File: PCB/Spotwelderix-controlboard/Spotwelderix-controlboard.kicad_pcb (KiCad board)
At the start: 2 copper layers, 83 x 60 mm, 42 parts, among them J2 LEDs, J3 Switch_OnOFF, J4 Int_Charger_supply, P1 Display, P2 CONN_01X08, Q1 DMG1012T-7, Q2 DMG1012T-7, Q3 DMG1012T-7, Q4 DMG1012T-7, U1 NodeMCU32, U2 ADS1115_Module, U3 LM7805M_TO263

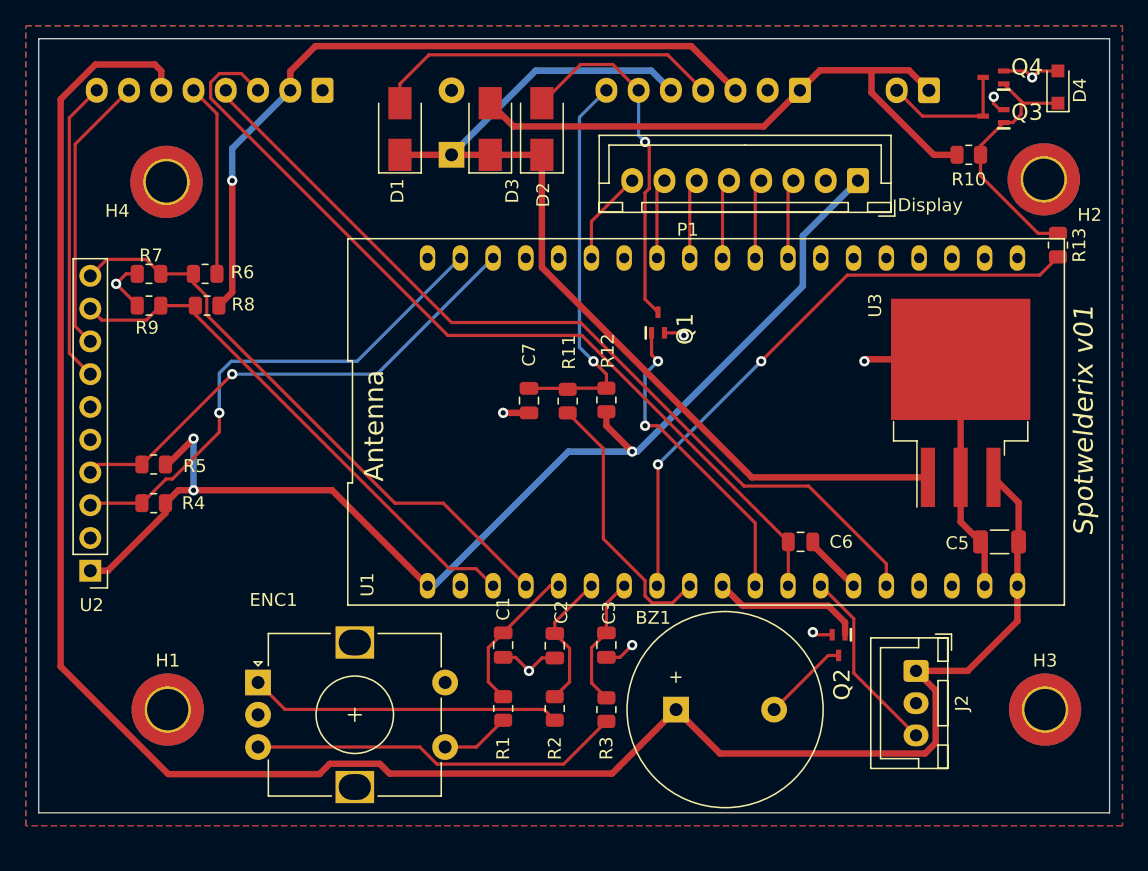
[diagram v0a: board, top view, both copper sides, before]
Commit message: ordered version v01
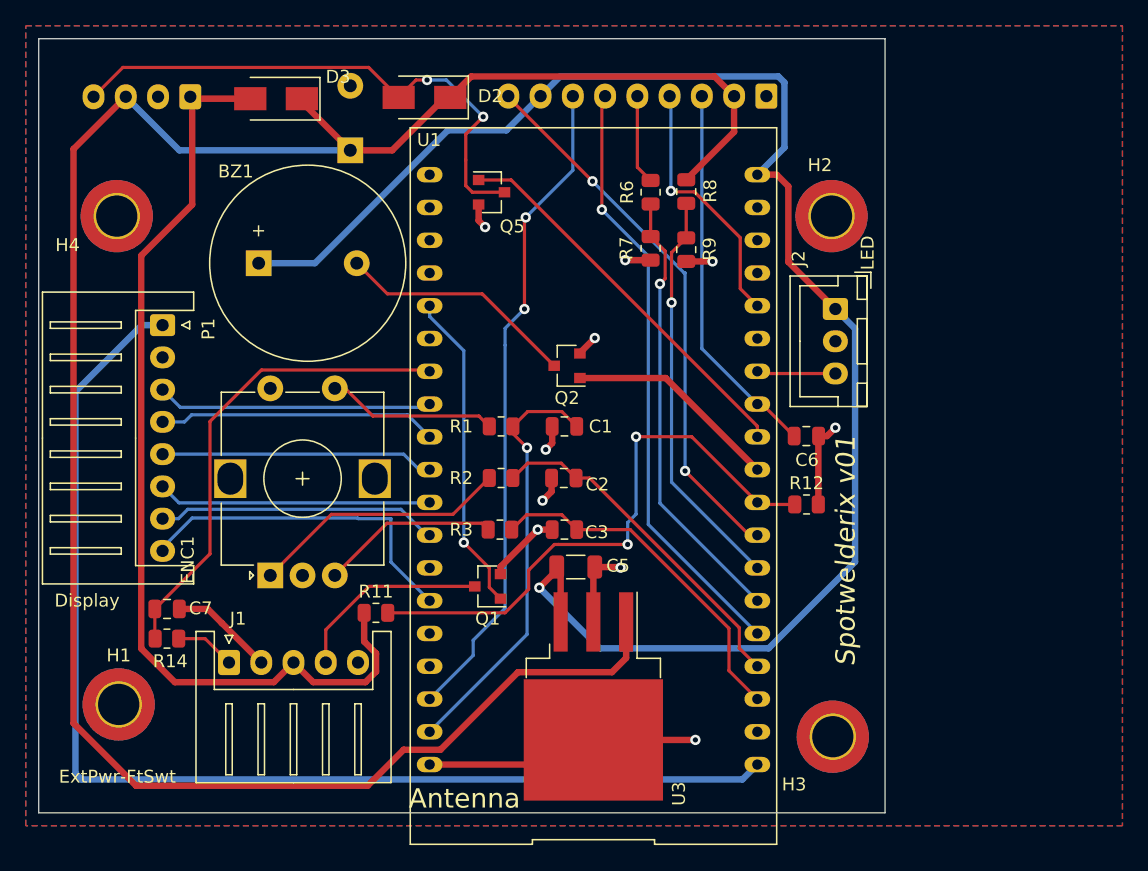
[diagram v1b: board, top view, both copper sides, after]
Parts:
- removed D1: D, Diode_SMD:D_SMA
- removed D4: 3.6V, Diode_SMD:D_SOD-323_HandSoldering
- removed J4: Int_Charger_supply, Connector_JST:JST_XH_B2B-XH-A_1x02_P2.50mm_Vertical
- removed Q3, Q4: DMG1012T-7, SamacSys_Parts:SOT50P160X80-3N
- removed R10: 10k, Resistor_SMD:R_0805_2012Metric
- removed R13: 100, Resistor_SMD:R_0805_2012Metric
- removed R4, R5: 3k3, Resistor_SMD:R_0805_2012Metric
- removed U2: ADS1115_Module, Connector_PinHeader_2.54mm:PinHeader_1x10_P2.54mm_Vertical
- added J1: ChargerPower, Connector_JST:JST_XH_S5B-XH-A_1x05_P2.50mm_Horizontal, F.Cu at (34.8, 68.3)
- added Q5: AO3400A, Package_TO_SOT_SMD:SOT-23, F.Cu at (55.1, 31.9)
- added R14: 100, Resistor_SMD:R_0805_2012Metric, F.Cu at (29.9, 66.5)
- C7: value 100n -> 100p
- J3: value Switch_OnOFF -> ExtPwr_FAn; footprint Connector_JST:JST_XH_B7B-XH-A_1x07_P2.50mm_Vertical -> Connector_JST:JST_XH_B4B-XH-A_1x04_P2.50mm_Vertical
- P1: footprint Connector_JST:JST_XH_B8B-XH-A_1x08_P2.50mm_Vertical -> Connector_JST:JST_XH_S8B-XH-A_1x08_P2.50mm_Horizontal
- P2: value CONN_01X08 -> PowerPCB; footprint Connector_JST:JST_XH_B8B-XH-A_1x08_P2.50mm_Vertical -> Connector_JST:JST_XH_B9B-XH-A_1x09_P2.50mm_Vertical
- Q1, Q2: value DMG1012T-7 -> AO3400A; footprint SamacSys_Parts:SOT50P160X80-3N -> Package_TO_SOT_SMD:SOT-23
- R11: value 100 -> 33k
- moved P1 55.1 mm to (29.6, 42.2), turned to 270 degrees
- moved BZ1 47.4 mm to (37.0, 37.4)
- moved J3 47.3 mm to (31.8, 24.5)
- moved R9 41.9 mm to (70.2, 36.3), turned to 270 degrees
- moved R7 38.9 mm to (67.4, 36.2), turned to 270 degrees
- moved R8 38.2 mm to (70.2, 31.8), turned to 270 degrees
- moved U3 36.4 mm to (63.0, 71.0), turned to 270 degrees
- moved R6 35.1 mm to (67.4, 31.9), turned to 270 degrees
- moved P2 34.4 mm to (76.4, 24.4)
- moved C5 32.9 mm to (61.6, 61.0), turned to 0 degrees
- moved C7 32.4 mm to (29.9, 64.2), turned to 0 degrees
- moved Q2 30.2 mm to (61.0, 45.4), turned to 180 degrees
- moved J2 28.7 mm to (81.8, 41.0)
- moved Q1 24.3 mm to (54.8, 62.5), turned to 180 degrees
- moved R11 22.1 mm to (46.1, 64.5), turned to 0 degrees
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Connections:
- C4 pad 1: /LM7805_in -> VCC
- C7 pad 1: Net-(C7-Pad1) -> FootSwitch
- D2 pad 1: /LM7805_in -> VCC
- D3 pad 1: /LM7805_in -> VCC
- J3 pad 4: Net-(D1-Pad2) -> FAN_GND
- P2 pad 6: +5V -> Vbat_ADC
- P2 pad 7: R_Schunt_H -> EnableSupply
- P2 pad 8: R_Schunt_L -> +5V
- Q1 pad 1: FAN -> ChargerEna
- Q1 pad 3: FAN_GND -> Net-(J1-Pad4)
- R11 pad 1: Net-(C7-Pad1) -> ExtPower
- R11 pad 2: Ext_Trigger -> ExtPWRADC
- R12 pad 1: +3V3 -> ExtPWRADC
- R12 pad 2: Net-(C7-Pad1) -> GND
- R6 pad 2: A3_VCC_ADC -> ProbeADC
- R7 pad 1: A3_VCC_ADC -> ProbeADC
- R8 pad 2: A2_ProbeADC -> VCC_ADC
- R9 pad 1: A2_ProbeADC -> VCC_ADC
- U1 pad 24: Net-(U1-Pad24) -> ChargerEna
- U1 pad 26: Net-(U1-Pad26) -> FootSwitch
- U1 pad 3: A2_ProbeADC -> UI_RotEnc_B
- U1 pad 36: SDA -> EnableSupply
- U1 pad 37: SCL -> UI_RotEnc_Push
- U1 pad 4: A3_VCC_ADC -> UI_RotEnc_A
- U1 pad 5: UI_RotEnc_Push -> Vbat_ADC
- U1 pad 6: UI_RotEnc_A -> ProbeADC
- U1 pad 7: UI_RotEnc_B -> VCC_ADC
- U1 pad 8: ChargDisEna -> Shuntvoltage
- U1 pad 9: Ext_Trigger -> ExtPWRADC
- U3 pad 1: /LM7805_in -> VCC
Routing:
- net VCC: track 57.2 -> 167.8 mm, vias 1 -> 0
- net /LM7805_in: track 76.7 -> 0.00 mm
- net EnableSupply: track 0.00 -> 51.3 mm, vias 0 -> 2
- net Dallas: track 68.4 -> 20.1 mm, vias 0 -> 1
- net ChargDisEna: track 47.1 -> 0.00 mm, vias 2 -> 0
- net Vbat_ADC: track 0.00 -> 46.7 mm, vias 0 -> 1
- net A3_VCC_ADC: track 46.0 -> 0.00 mm
- net ExtPWRADC: track 0.00 -> 44.7 mm, vias 0 -> 2
- net Shuntvoltage: track 0.00 -> 42.4 mm, vias 0 -> 2
- net A2_ProbeADC: track 41.5 -> 0.00 mm
- net SCL: track 39.3 -> 0.00 mm, vias 1 -> 0
- net Gate_logic: track 68.1 -> 29.5 mm
- net SDA: track 38.1 -> 0.00 mm, vias 1 -> 0
- net FootSwitch: track 0.00 -> 37.4 mm
- net ProbeADC: track 0.00 -> 34.5 mm, vias 0 -> 1
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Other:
- board size 83 x 60 mm -> 65.6 x 60 mm
- board text added: "ExtPwr-FtSwt"
- board text added: "LED"

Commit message: ordered seperately
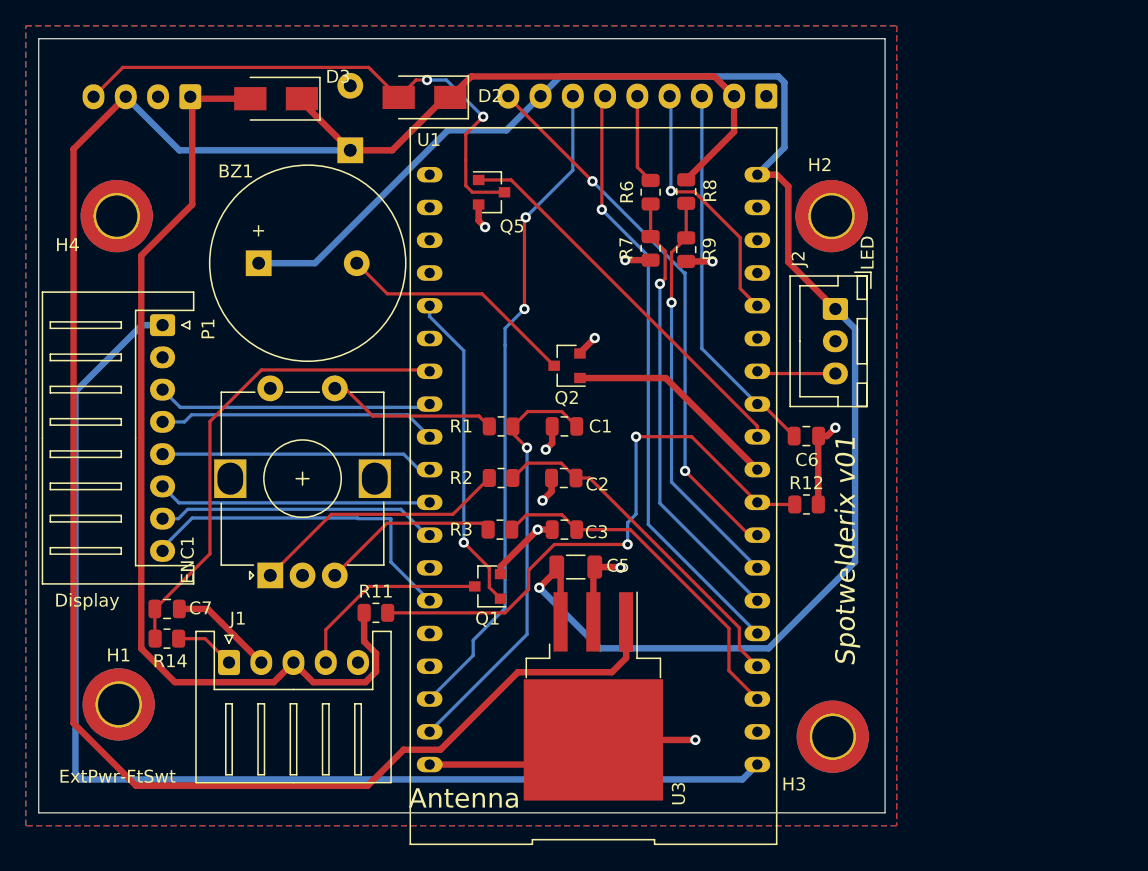
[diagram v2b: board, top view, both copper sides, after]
